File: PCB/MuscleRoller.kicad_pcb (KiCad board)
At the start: 2 copper layers, 83 x 71 mm, 52 parts, among them J1 Conn_01x06_Male, J10 Conn_01x06_Male, J11 Conn_01x06_Male, J12 Conn_01x06_Male, J13 Conn_02x03_Odd_Even, J14 Conn_02x03_Odd_Even, J15 Conn_02x03_Odd_Even, J16 Conn_01x04_Male, J17 Conn_01x04_Male, J18 Conn_01x04_Male, J19 Conn_01x04_Male, J2 Conn_01x06_Male, J3 Screw_Terminal_01x02, J4 Conn_02x03_Odd_Even, J5 Conn_02x03_Odd_Even, J6 Conn_01x03_Male, J7 Conn_01x04_Male, J8 Conn_01x04_Male, J9 Conn_01x02_Male, U1 AZ1117-3.3, U2 ESP32-S2-WROOM, U3 ZXBM5210-S, U4 TB67H451FNG,EL

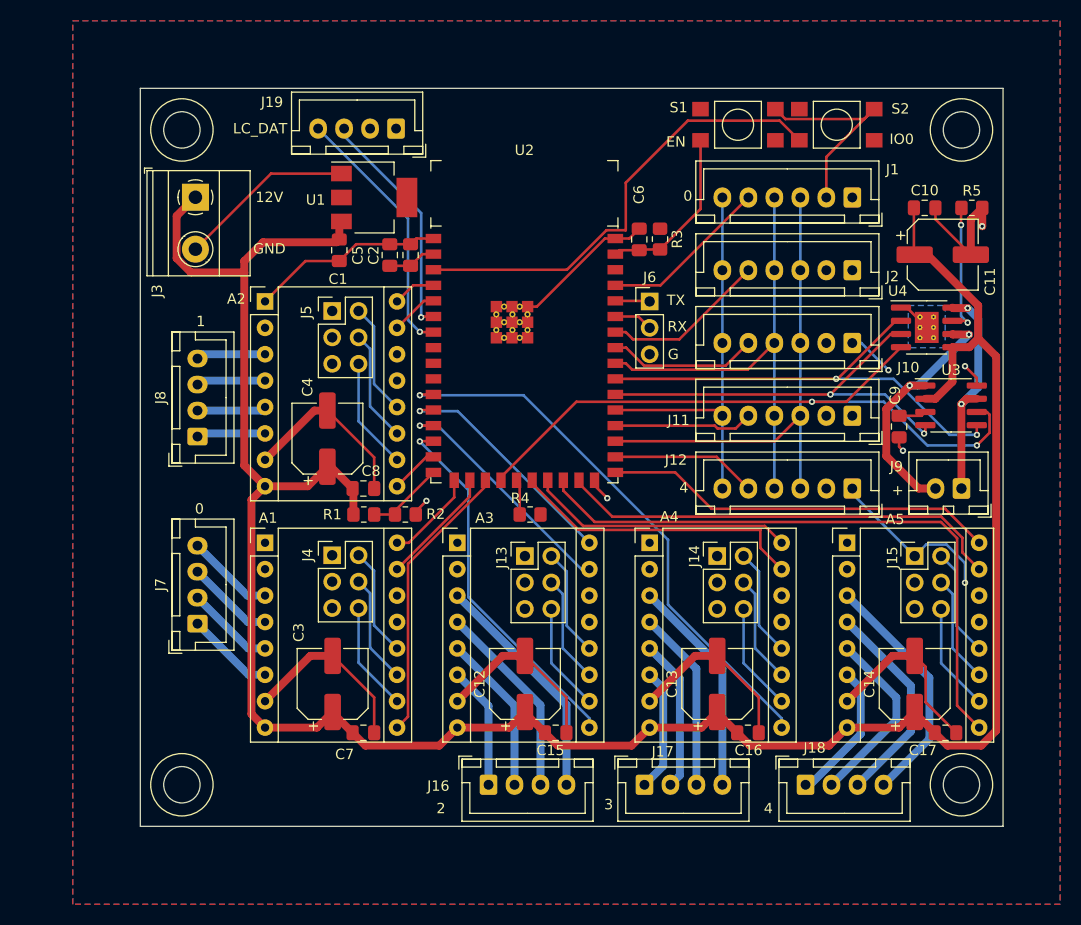
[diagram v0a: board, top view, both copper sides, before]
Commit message: PCB complete
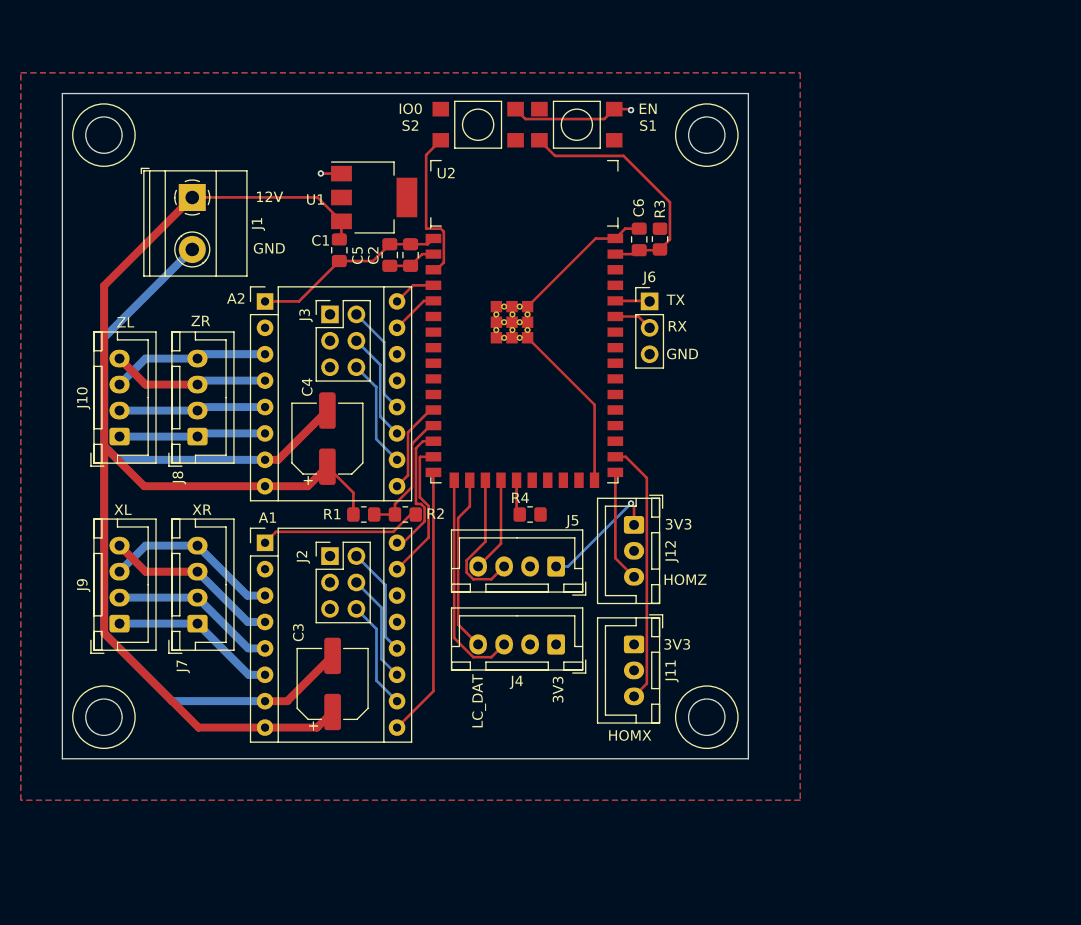
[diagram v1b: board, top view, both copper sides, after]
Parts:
- removed A3, A4, A5: Pololu_Breakout_DRV8825, Module:Pololu_Breakout-16_15.2x20.3mm
- removed C10: 0.1U, Capacitor_SMD:C_0805_2012Metric_Pad1.18x1.45mm_HandSolder
- removed C11: 100U, Capacitor_SMD:CP_Elec_6.3x7.7
- removed C12, C13, C14: 100u, Capacitor_SMD:CP_Elec_6.3x7.7
- removed C15, C16, C17, C7, C8: 0.1u, Capacitor_SMD:C_0805_2012Metric_Pad1.18x1.45mm_HandSolder
- removed C9: 1U, Capacitor_SMD:C_0805_2012Metric_Pad1.18x1.45mm_HandSolder
- removed J13, J14, J15: Conn_02x03_Odd_Even, Connector_PinHeader_2.54mm:PinHeader_2x03_P2.54mm_Vertical
- removed J16, J17, J18, J19: Conn_01x04_Male, Connector_JST:JST_XH_B4B-XH-A_1x04_P2.50mm_Vertical
- removed R5: 0.1, Resistor_SMD:R_0805_2012Metric_Pad1.20x1.40mm_HandSolder
- removed U3: ZXBM5210-S, Package_SO:SOIC-8_3.9x4.9mm_P1.27mm
- removed U4: TB67H451FNG,EL, Package_SO:SOIC-8-1EP_3.9x4.9mm_P1.27mm_EP2.29x3mm_ThermalVias
- J1: value Conn_01x06_Male -> Screw_Terminal_01x02; footprint Connector_JST:JST_XH_B6B-XH-A_1x06_P2.50mm_Vertical -> TerminalBlock_Phoenix:TerminalBlock_Phoenix_MKDS-1,5-2_1x02_P5.00mm_Horizontal
- J10: value Conn_01x06_Male -> Conn_01x04_Male; footprint Connector_JST:JST_XH_B6B-XH-A_1x06_P2.50mm_Vertical -> Connector_JST:JST_XH_B4B-XH-A_1x04_P2.50mm_Vertical
- J11, J12: value Conn_01x06_Male -> Conn_01x03_Male; footprint Connector_JST:JST_XH_B6B-XH-A_1x06_P2.50mm_Vertical -> Connector_JST:JST_XH_B3B-XH-A_1x03_P2.50mm_Vertical
- J2: value Conn_01x06_Male -> Conn_02x03_Odd_Even; footprint Connector_JST:JST_XH_B6B-XH-A_1x06_P2.50mm_Vertical -> Connector_PinHeader_2.54mm:PinHeader_2x03_P2.54mm_Vertical
- J3: value Screw_Terminal_01x02 -> Conn_02x03_Odd_Even; footprint TerminalBlock_Phoenix:TerminalBlock_Phoenix_MKDS-1,5-2_1x02_P5.00mm_Horizontal -> Connector_PinHeader_2.54mm:PinHeader_2x03_P2.54mm_Vertical
- J4, J5: value Conn_02x03_Odd_Even -> Conn_01x04_Male; footprint Connector_PinHeader_2.54mm:PinHeader_2x03_P2.54mm_Vertical -> Connector_JST:JST_XH_B4B-XH-A_1x04_P2.50mm_Vertical
- J9: value Conn_01x02_Male -> Conn_01x04_Male; footprint Connector_JST:JST_XH_B2B-XH-A_1x02_P2.50mm_Vertical -> Connector_JST:JST_XH_B4B-XH-A_1x04_P2.50mm_Vertical
- R4: value 47K -> 10K
- moved J9 82.0 mm to (59.5, 103.0), turned to 90 degrees
- moved J10 71.1 mm to (59.5, 85.0), turned to 90 degrees
- moved J1 63.5 mm to (66.5, 62.0), turned to 270 degrees
- moved J2 57.3 mm to (79.8, 96.5), turned to 0 degrees
- moved S2 34.5 mm to (94.0, 55.0)
- moved J5 32.7 mm to (101.5, 97.5), turned to 180 degrees
- moved J11 30.4 mm to (109.0, 105.0), turned to 270 degrees
- moved J4 23.2 mm to (101.5, 105.0), turned to 180 degrees
- moved J12 21.3 mm to (109.0, 93.5), turned to 270 degrees
- moved J3 17.2 mm to (79.8, 73.2), turned to 0 degrees
- moved S1 15.5 mm to (103.5, 55.0)
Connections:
- net DIR1 renamed DIRZ
- net STEP1 renamed STEPZ
- A1 pad 15: STEP0 -> STEPX
- A1 pad 16: DIR0 -> DIRX
- A1 pad 3: Net-(A1-Pad3) -> XA2
- A1 pad 4: Net-(A1-Pad4) -> XA1
- A1 pad 5: Net-(A1-Pad5) -> XB1
- A1 pad 6: Net-(A1-Pad6) -> XB2
- A1 pad 9: EN0 -> ENX
- A2 pad 3: Net-(A2-Pad3) -> ZA2
- A2 pad 4: Net-(A2-Pad4) -> ZA1
- A2 pad 5: Net-(A2-Pad5) -> ZB1
- A2 pad 6: Net-(A2-Pad6) -> ZB2
- A2 pad 9: EN1 -> ENZ
- J1 pad 1: +3V3 -> +12V
- J10 pad 1: +3V3 -> ZB2
- J10 pad 2: GND -> ZB1
- J10 pad 3: CLK -> ZA2
- J10 pad 4: MISO -> ZA1
- J11 pad 3: CLK -> HOMX
- J12 pad 3: CLK -> HOMZ
- J2 pad 2: GND -> Net-(A1-Pad12)
- J2 pad 3: CLK -> +3V3
- J2 pad 4: MISO -> Net-(A1-Pad11)
- J2 pad 5: CS1 -> +3V3
- J2 pad 6: MOSI -> Net-(A1-Pad10)
- J3 pad 1: +12V -> +3V3
- J3 pad 2: GND -> Net-(A2-Pad12)
- J4 pad 2: Net-(A1-Pad12) -> GND
- J4 pad 3: +3V3 -> LC_CLK
- J4 pad 4: Net-(A1-Pad11) -> LC_DAT
- J5 pad 2: Net-(A2-Pad12) -> GND
- J5 pad 3: +3V3 -> LC_CLK2
- J5 pad 4: Net-(A2-Pad11) -> LC_DAT2
- J7 pad 1: Net-(A1-Pad6) -> XB2
- J7 pad 2: Net-(A1-Pad5) -> XB1
- J7 pad 3: Net-(A1-Pad4) -> XA1
- J7 pad 4: Net-(A1-Pad3) -> XA2
- J8 pad 1: Net-(A2-Pad6) -> ZB2
- J8 pad 2: Net-(A2-Pad5) -> ZB1
- J8 pad 3: Net-(A2-Pad4) -> ZA1
- J8 pad 4: Net-(A2-Pad3) -> ZA2
- J9 pad 1: OUT2 -> XB2
- J9 pad 2: OUT1 -> XB1
- U2 pad 11: EN3 -> Net-(U2-Pad11)
- U2 pad 12: DIR2 -> ENZ
- U2 pad 13: STEP2 -> CHARGE
- U2 pad 14: EN2 -> DIRX
- U2 pad 15: EN1 -> STEPX
- U2 pad 16: CHARGE -> ENX
- U2 pad 17: DIR0 -> LC_CLK
- U2 pad 18: STEP0 -> LC_DAT
- U2 pad 19: EN0 -> LC_CLK2
- U2 pad 20: DAC1 -> LC_DAT2
- U2 pad 22: STEP3 -> Net-(U2-Pad22)
- U2 pad 23: DIR3 -> Net-(U2-Pad23)
- U2 pad 24: EN4 -> Net-(U2-Pad24)
- U2 pad 25: STEP4 -> Net-(U2-Pad25)
- U2 pad 27: DIR4 -> HOMZ
- U2 pad 28: CS4 -> HOMX
- U2 pad 29: CLK -> Net-(U2-Pad29)
- U2 pad 30: CS3 -> Net-(U2-Pad30)
- U2 pad 31: MOSI -> Net-(U2-Pad31)
- U2 pad 32: MOT1 -> Net-(U2-Pad32)
- U2 pad 33: MOT2 -> Net-(U2-Pad33)
- U2 pad 34: MISO -> Net-(U2-Pad34)
- U2 pad 35: CS2 -> Net-(U2-Pad35)
- U2 pad 36: CS1 -> Net-(U2-Pad36)
- U2 pad 39: CS0 -> Net-(U2-Pad39)
- U2 pad 6: LC_CLK -> Net-(U2-Pad6)
- U2 pad 7: LC_DAT -> Net-(U2-Pad7)
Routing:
- net +12V: track 230.2 -> 118.4 mm
- net DAC1: track 66.4 -> 0.00 mm, vias 2 -> 0
- net EN4: track 59.9 -> 0.00 mm
- net EN3: track 53.6 -> 0.00 mm, vias 1 -> 0
- net CLK: track 46.8 -> 0.00 mm
- net MOT2: track 46.5 -> 0.00 mm, vias 2 -> 0
- net MISO: track 44.6 -> 0.00 mm
- net STEP4: track 43.0 -> 0.00 mm
- net MOT1: track 41.3 -> 0.00 mm, vias 2 -> 0
- net MOSI: track 38.5 -> 0.00 mm
- net DIR4: track 37.8 -> 0.00 mm
- net EN2: track 35.6 -> 0.00 mm, vias 1 -> 0
- net IO0: track 44.6 -> 15.2 mm
- net STEP3: track 28.7 -> 0.00 mm
- net EN0: track 27.3 -> 0.00 mm
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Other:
- board size 83 x 71 mm -> 66 x 64 mm
- board text added: "3V3"
- board text added: "HOMX"
- board text added: "HOMZ"
- board text added: "XL"
- board text added: "XR"
- board text added: "ZL"
- board text added: "ZR"
- board text removed: "+"
- board text removed: "0"
- board text removed: "1"
- board text removed: "2"
- board text removed: "3"
- board text removed: "4"
- board text removed: "G"
- board text removed: "SAGE ROBOTS A4 2.0"
